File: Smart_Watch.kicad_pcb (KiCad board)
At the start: 4 copper layers, 32 x 32 mm, 59 parts, among them J1 USB_C_Receptacle, J2 Conn_01x02, J3 Conn_01x06, J4 Conn_01x02, SW2 SW_Push, SW3 SW_Push, SW4 SW_Push, SW5 SW_Push, SW6 SW_Push, SW7 SW_Push, U1 MAX30102, U10 DRV2603RUNR, U11 ESDR0502NMUTBG, U2 BMI270, U3 OPT3004DNPR, U4 LPS22DF, U5 W25Q32JVSS, U6 NPM1300-QEAA-R7, U8 FAN5622SX, U9 NORA-B106-00B, X1 Q13FC1350000400, X608 Display

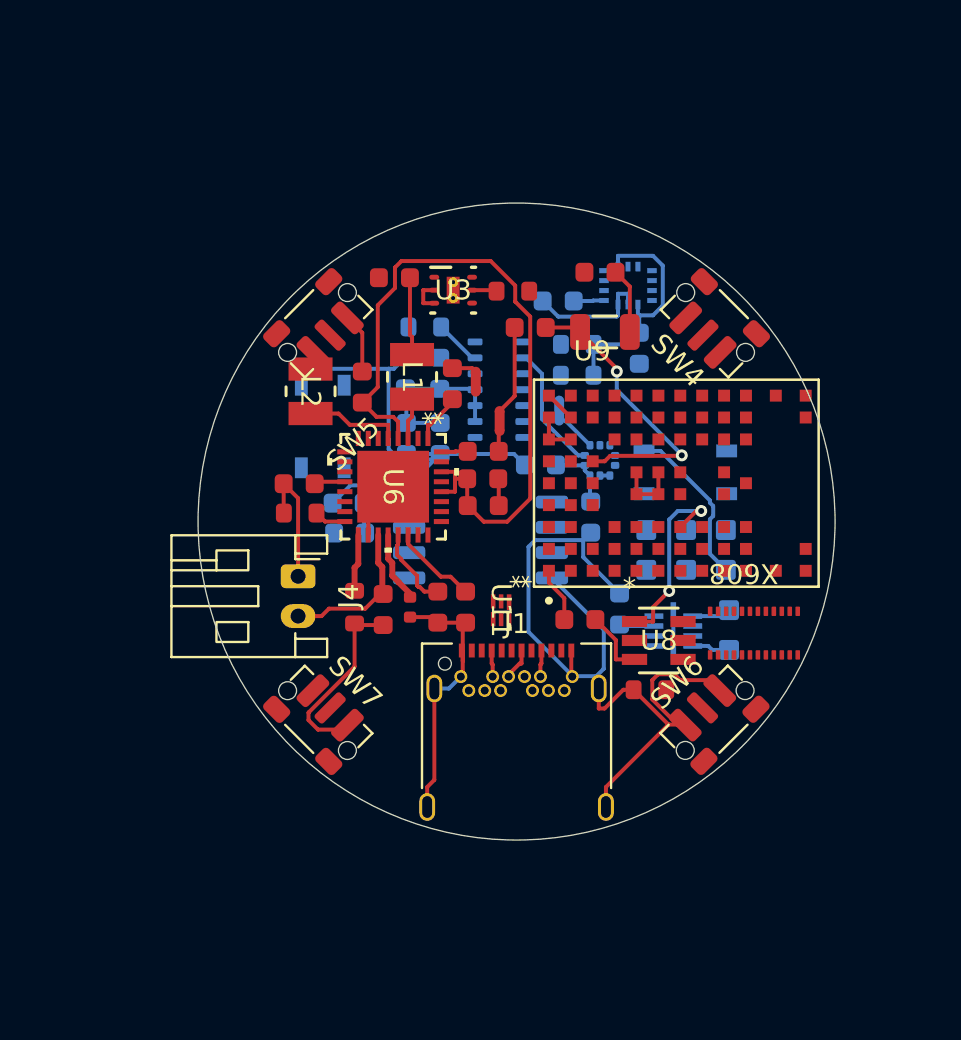
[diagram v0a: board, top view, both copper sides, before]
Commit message: I hate you git
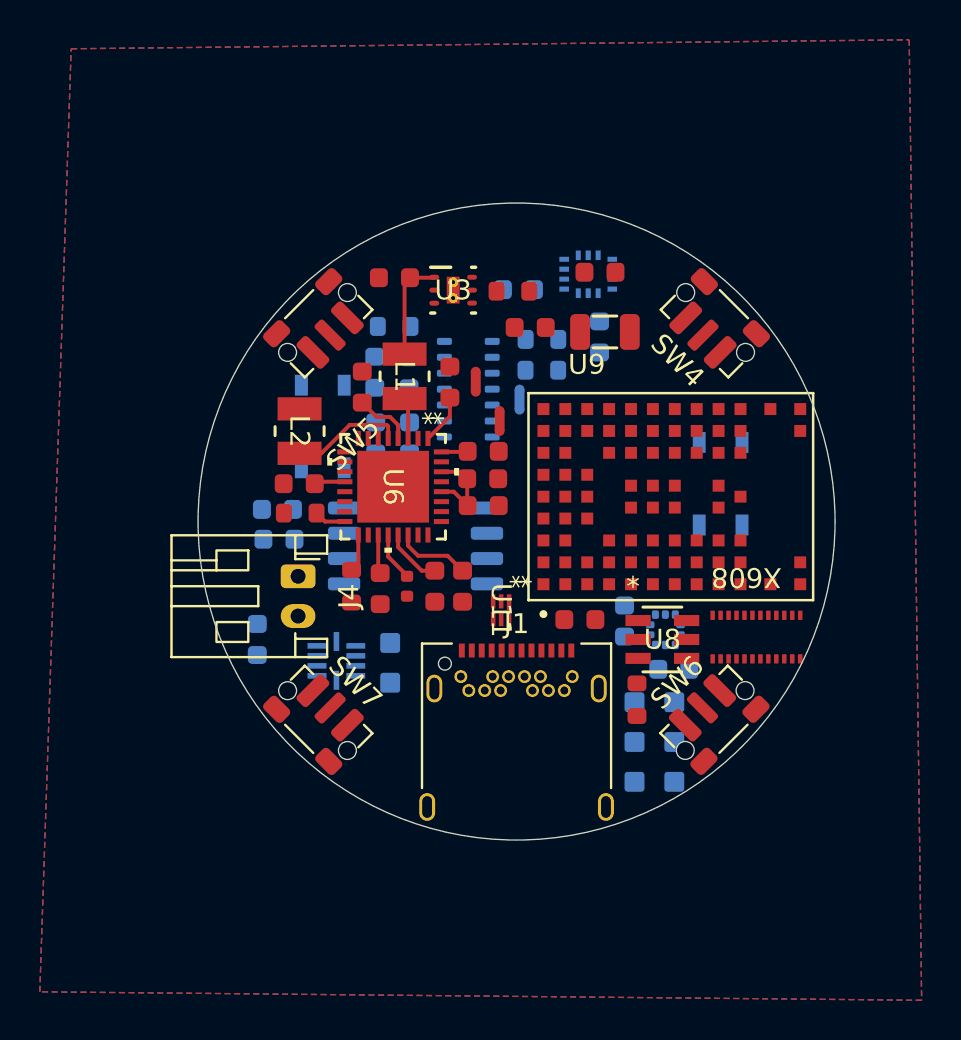
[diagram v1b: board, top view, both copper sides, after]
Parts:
- moved C23 18.3 mm to (159.1, 113.8)
- moved J2 17.1 mm to (165.8, 115.0)
- moved U10 17.0 mm to (163.1, 114.9)
- moved C9 12.3 mm to (180.1, 115.3), turned to 0 degrees
- moved J3 9.78 mm to (179.1, 118.9), turned to -90 degrees
- moved U4 9.12 mm to (179.6, 113.3)
- moved C8 5.49 mm to (177.6, 112.8), turned to 90 degrees
- moved C26 3.57 mm to (160.1, 107.2)
- moved C21 3.57 mm to (160.2, 108.7)
- moved U5 3.28 mm to (167.1, 109.1)
- moved C5 2.08 mm to (176.3, 98.6)
- moved C6 2.08 mm to (172.2, 96.2)
- moved U2 2.08 mm to (175.8, 95.4)
- moved L2 2.07 mm to (161.2, 103.3)
- moved NT3 2.06 mm to (172.3, 101.7)
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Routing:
- net GND: track 130.2 -> 0.00 mm
- net VSYS: track 41.9 -> 9.82 mm
- net +1V8: track 39.5 -> 9.24 mm
- net /Architecture/MCU/CLK1: track 14.7 -> 0.00 mm, vias 2 -> 0
- net /Architecture/MCU/DISPLAY_LIGHT_IO: track 9.56 -> 0.00 mm, vias 2 -> 0
- net /Architecture/MCU/MCU_RST: track 8.30 -> 0.00 mm
- net /Architecture/MCU/SCL: track 6.47 -> 0.00 mm
- net +BATT: track 7.81 -> 1.96 mm
- net /Architecture/MCU/VBUS_IN: track 6.81 -> 2.94 mm
- net +3V0: track 4.69 -> 1.33 mm
- net /Architecture/MCU/CLK2: track 3.30 -> 0.00 mm
- net /Architecture/MCU/MAX_INT: track 2.35 -> 0.00 mm
- net /Architecture/Peripherals/MOTOR-: track 1.95 -> 0.00 mm
- net /Architecture/Peripherals/MOTOR+: track 1.91 -> 0.00 mm
- net /Architecture/MCU/USBC_D-: track 1.63 -> 0.00 mm
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- added copper zone on B.Cu, net GND
- added copper zone on F.Cu, net GND
- added copper zone on In1.Cu, net GND
- added copper zone on In2.Cu, net GND
